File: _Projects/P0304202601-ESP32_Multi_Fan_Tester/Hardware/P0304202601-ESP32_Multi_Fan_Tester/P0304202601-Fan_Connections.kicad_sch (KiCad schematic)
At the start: 7 parts, among them CN1 KHS4B-PH-SM4-TB(LF)(SN), CN4 KTBL002B-350-04GR-2OR, CN5 KH470533000, J1 KH22-28-5021, J2 KH22-28-5021, J3 KH22-28-5021

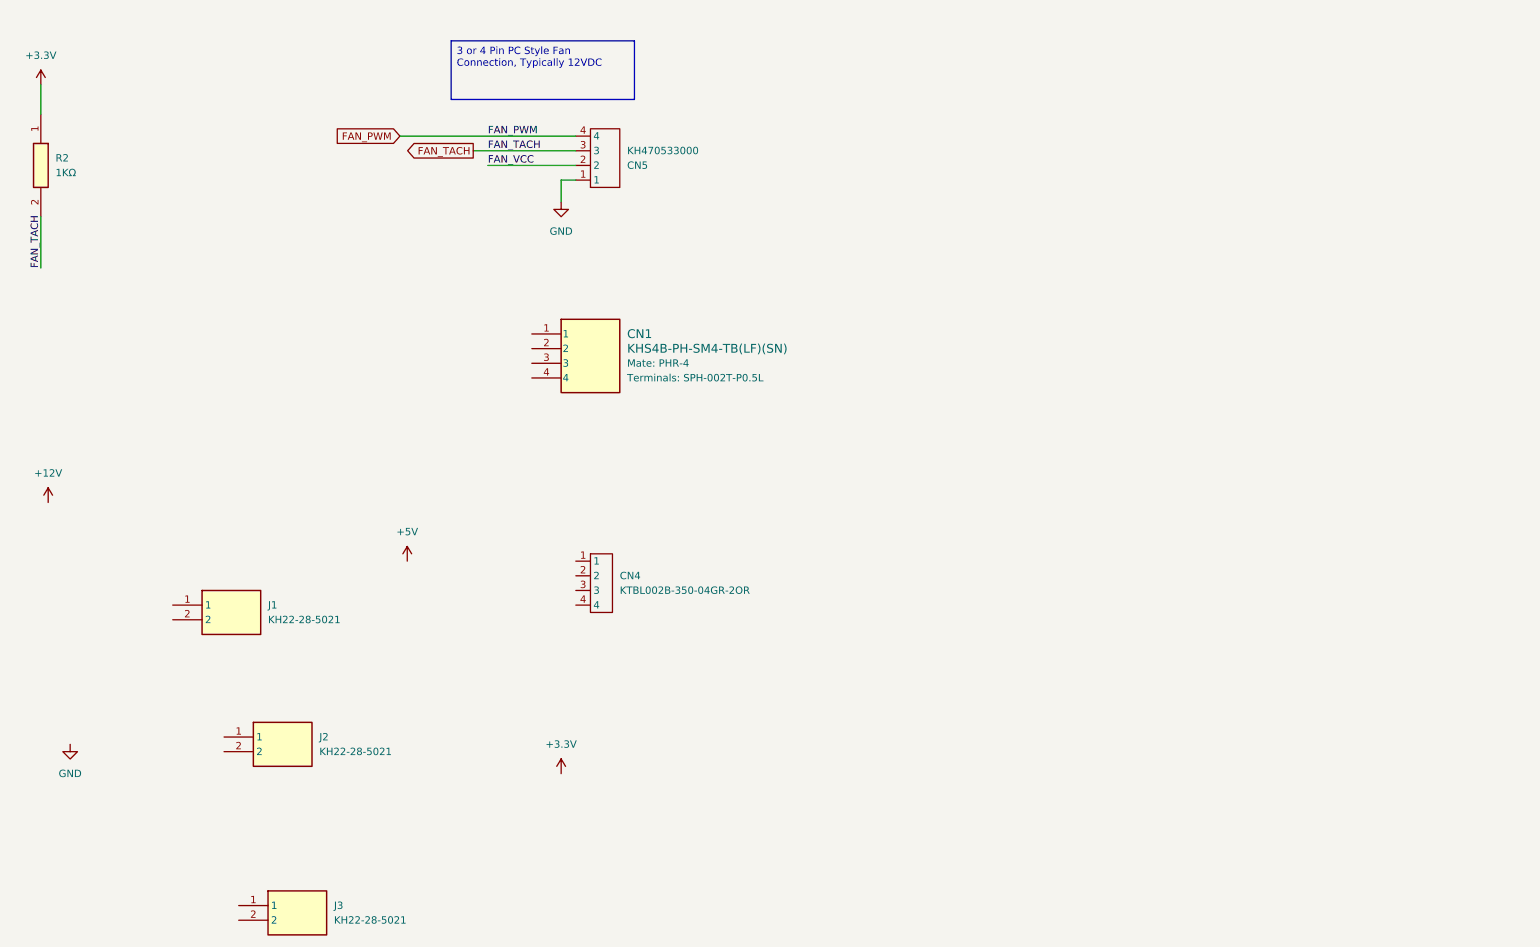
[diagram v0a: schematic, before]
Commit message: Added updated content that I keep forgetting to do.
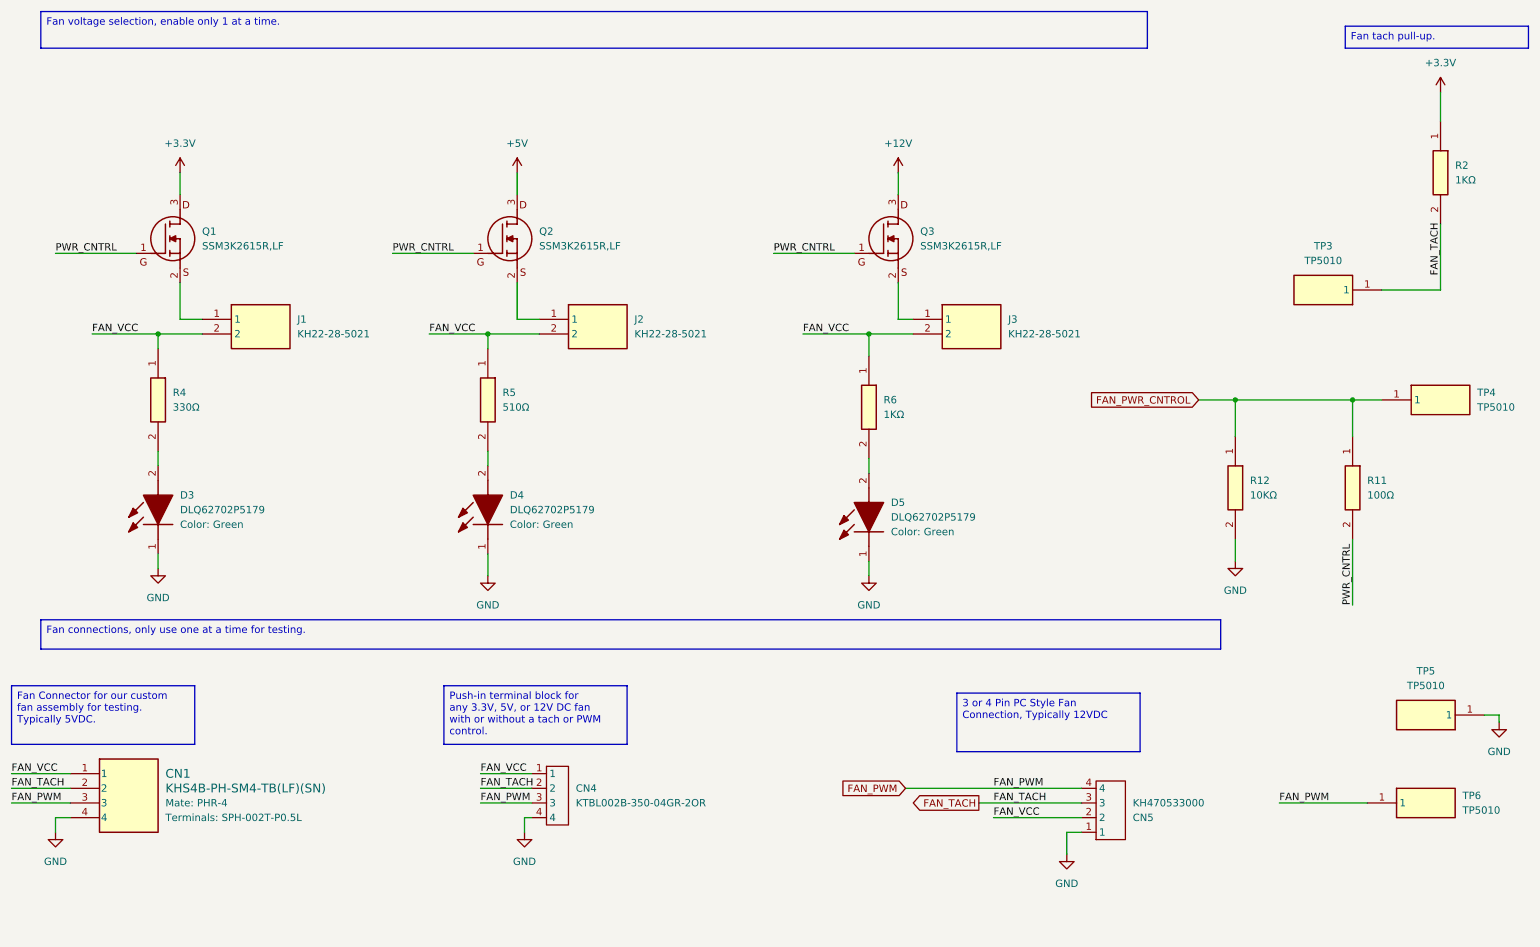
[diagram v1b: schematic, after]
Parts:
- added D3, D4, D5: DLQ62702P5179, COMPONENTS:LED-0805, symbol COMPONENTS:DLQ62702P5179
- added Q1, Q2, Q3: SSM3K2615R,LF, COMPONENTS:SOT-23F-3, symbol COMPONENTS:QSSM3K2615R,LF
- added R11: 100Ω, COMPONENTS:RES-0603, symbol COMPONENTS:RC0603100RAAD07500
- added R12: RC060310K2075AAA, COMPONENTS:RES-0603, symbol COMPONENTS:RC060310K2075AAA
- added R4: RC0603330075AAA, COMPONENTS:RES-0603, symbol COMPONENTS:RC0603330075AAA
- added R5: RC0603510075AAA, COMPONENTS:RES-0603, symbol COMPONENTS:RC0603510075AAA
- added R6: RC06031K0075AAA, COMPONENTS:RES-0603, symbol COMPONENTS:RC06031K0075AAA
- added TP3, TP4, TP5, TP6: TP5010, CONNECTORS:5010, symbol CONNECTORS:TP5010
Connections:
- net +12V: now also Q3.3 (D)
- net +3.3V: now also Q1.3 (D)
- net +5V: now also Q2.3 (D)
- net FAN_PWM: now also CN1.3, CN4.3, TP6.1
- net FAN_TACH: now also CN1.2, CN4.2, TP3.1
- net FAN_VCC: now also CN1.1, CN4.1, J1.2, J2.2, J3.2, R4.1, R5.1, R6.1
- net GND: now also CN1.4, CN4.4, D3.1 (K), D4.1 (K), D5.1 (K), R12.2, TP5.1
- net at J2.1: now also Q2.2 (S)
- net at J3.1: now also Q3.2 (S)
- net at J1.1: now also Q1.2 (S)
- new net: D5.2 (A), R6.2
- new net: D3.2 (A), R4.2
- new net: D4.2 (A), R5.2
- new net FAN_PWR_CNTROL: R11.1, R12.1, TP4.1
- new net PWR_CNTRL: Q1.1 (G), Q2.1 (G), Q3.1 (G), R11.2
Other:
- moved on the sheet: CN1, CN4, CN5, J1, J2, J3, R2
